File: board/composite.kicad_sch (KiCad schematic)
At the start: 24 parts, among them J10 VGA, J5 VIDEO_JTAG_BYPASS, J6 COMPOSITE, U17 VIDEO, Y1 14.318MHz, Y3 25.175MHz

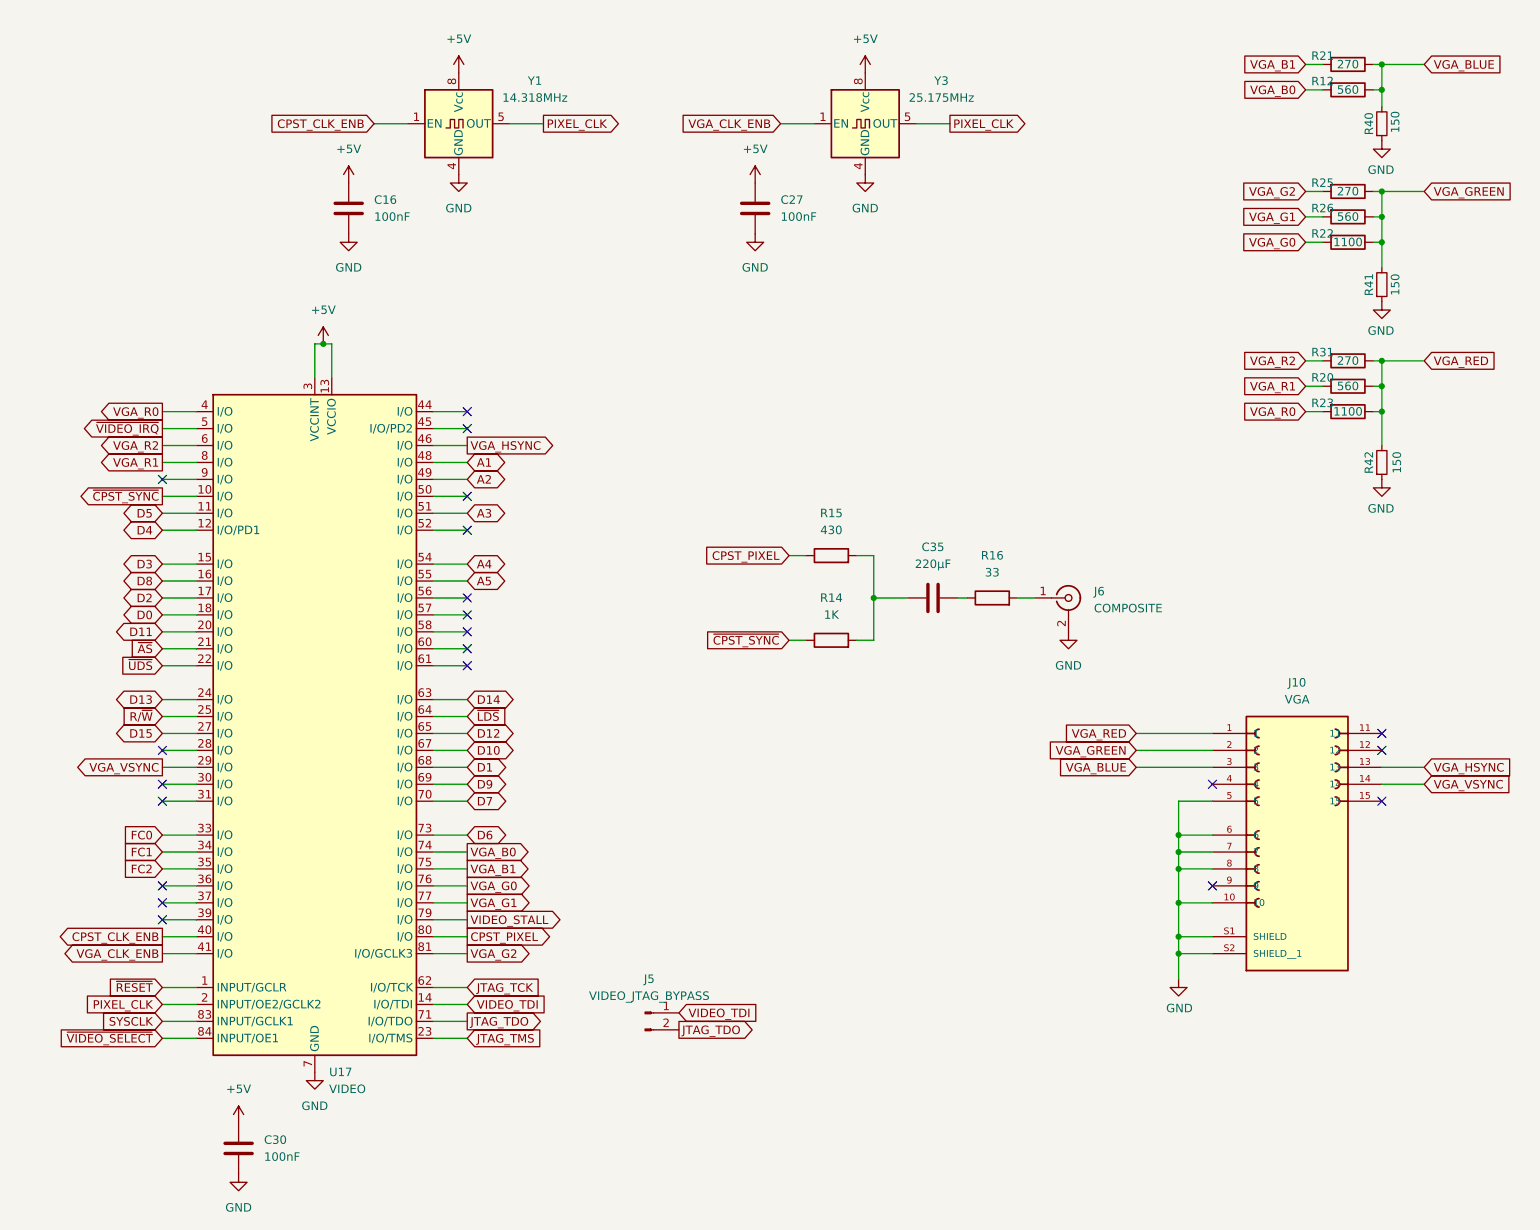
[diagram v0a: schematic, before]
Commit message: update parts I've added
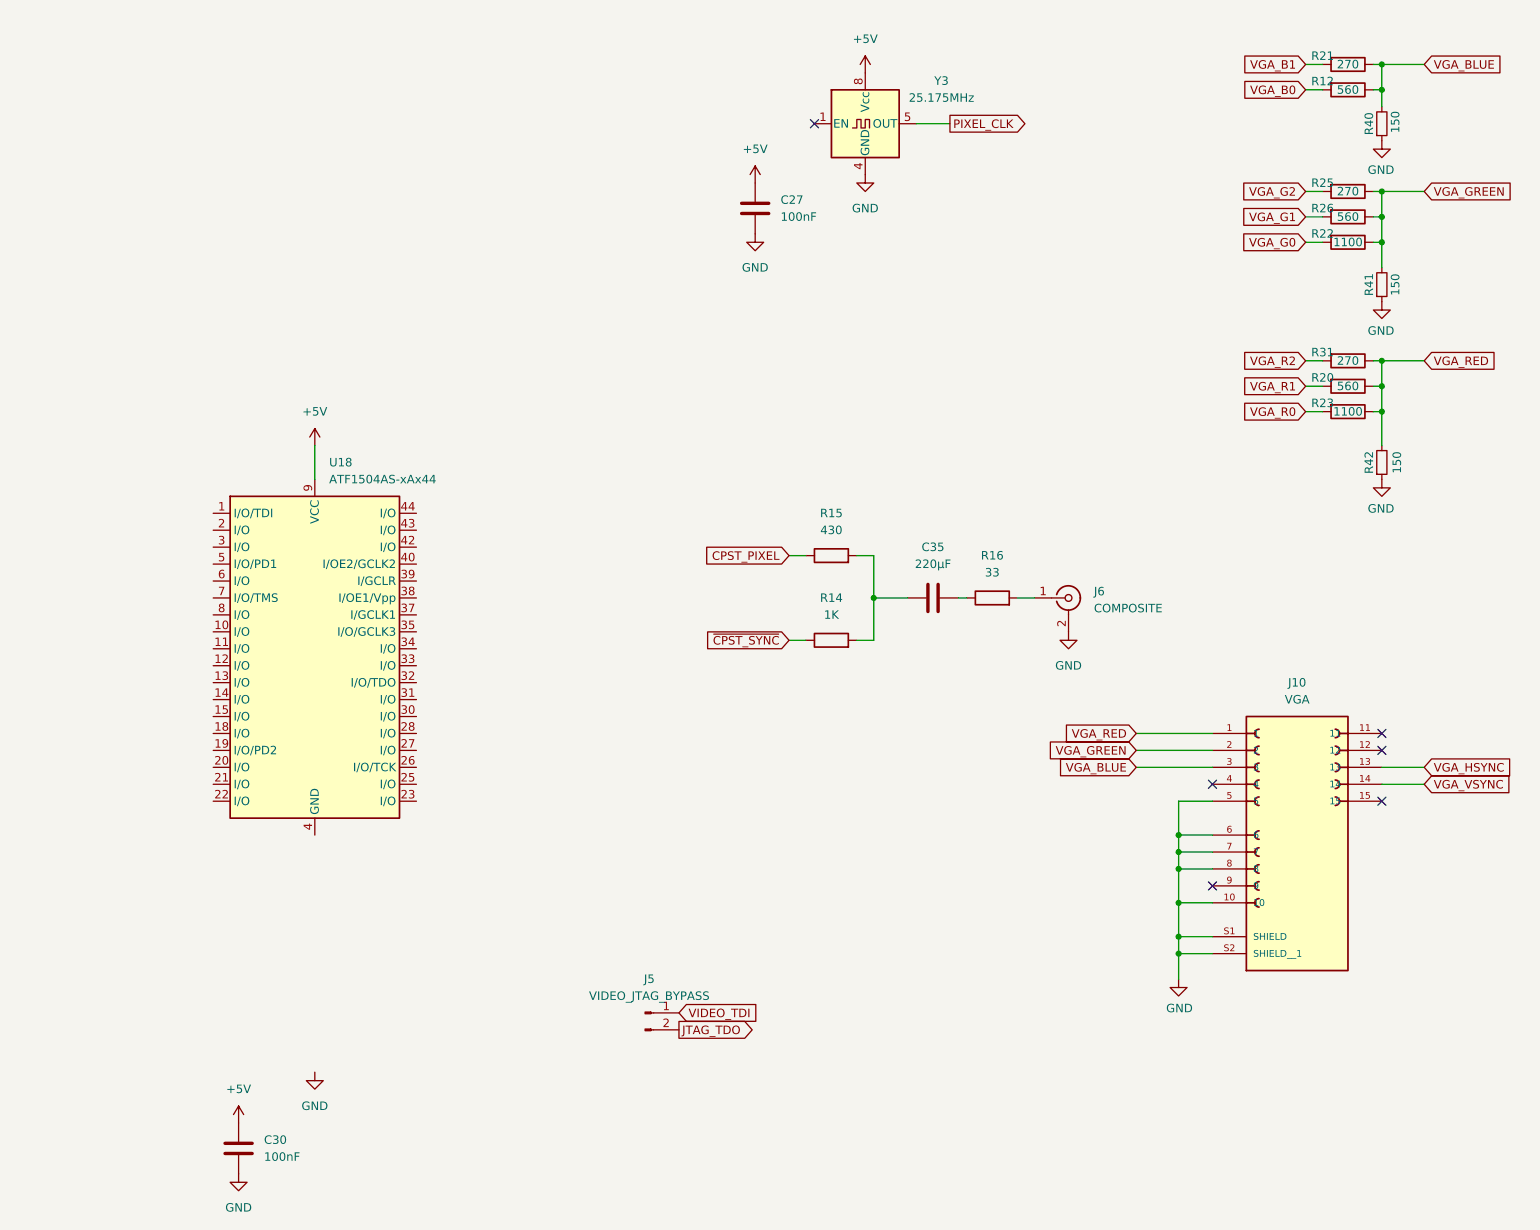
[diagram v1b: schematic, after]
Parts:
- removed C16: 100nF, Capacitor_THT:C_Disc_D5.0mm_W2.5mm_P5.00mm, symbol Device:C
- removed U17: VIDEO, Package_LCC:PLCC-84_THT-Socket, symbol CPLD_Microchip:ATF1508ASx-xxJx84
- removed Y1: 14.318MHz, Oscillator:Oscillator_DIP-8, symbol Oscillator:CXO_DIP8
- added U18: ATF1504AS-xAx44, Package_QFP:TQFP-44_10x10mm_P0.8mm, symbol CPLD_Microchip:ATF1504AS-xAx44
- Y3: Datasheet-rev1 (none) -> http://cdn-reichelt.de/documents/datenblatt/B400/OSZI.pdf; Digikey https://www.digikey.com/en/products/detail/shenzhen-sctf-el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 -> https://www.digikey.com/en/products/detail/ecs-inc/ECS-100A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
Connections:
- net +5V: now also U18.17 (VCC), U18.29 (VCC), U18.41 (VCC), U18.9 (VCC)
- net VGA_CLK_ENB: no longer names the net of Y3.1 (EN)
- new net: U18.16 (GND), U18.24 (GND), U18.36 (GND), U18.4 (GND)
- no-connect marks 21 -> 6

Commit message: checkpoint
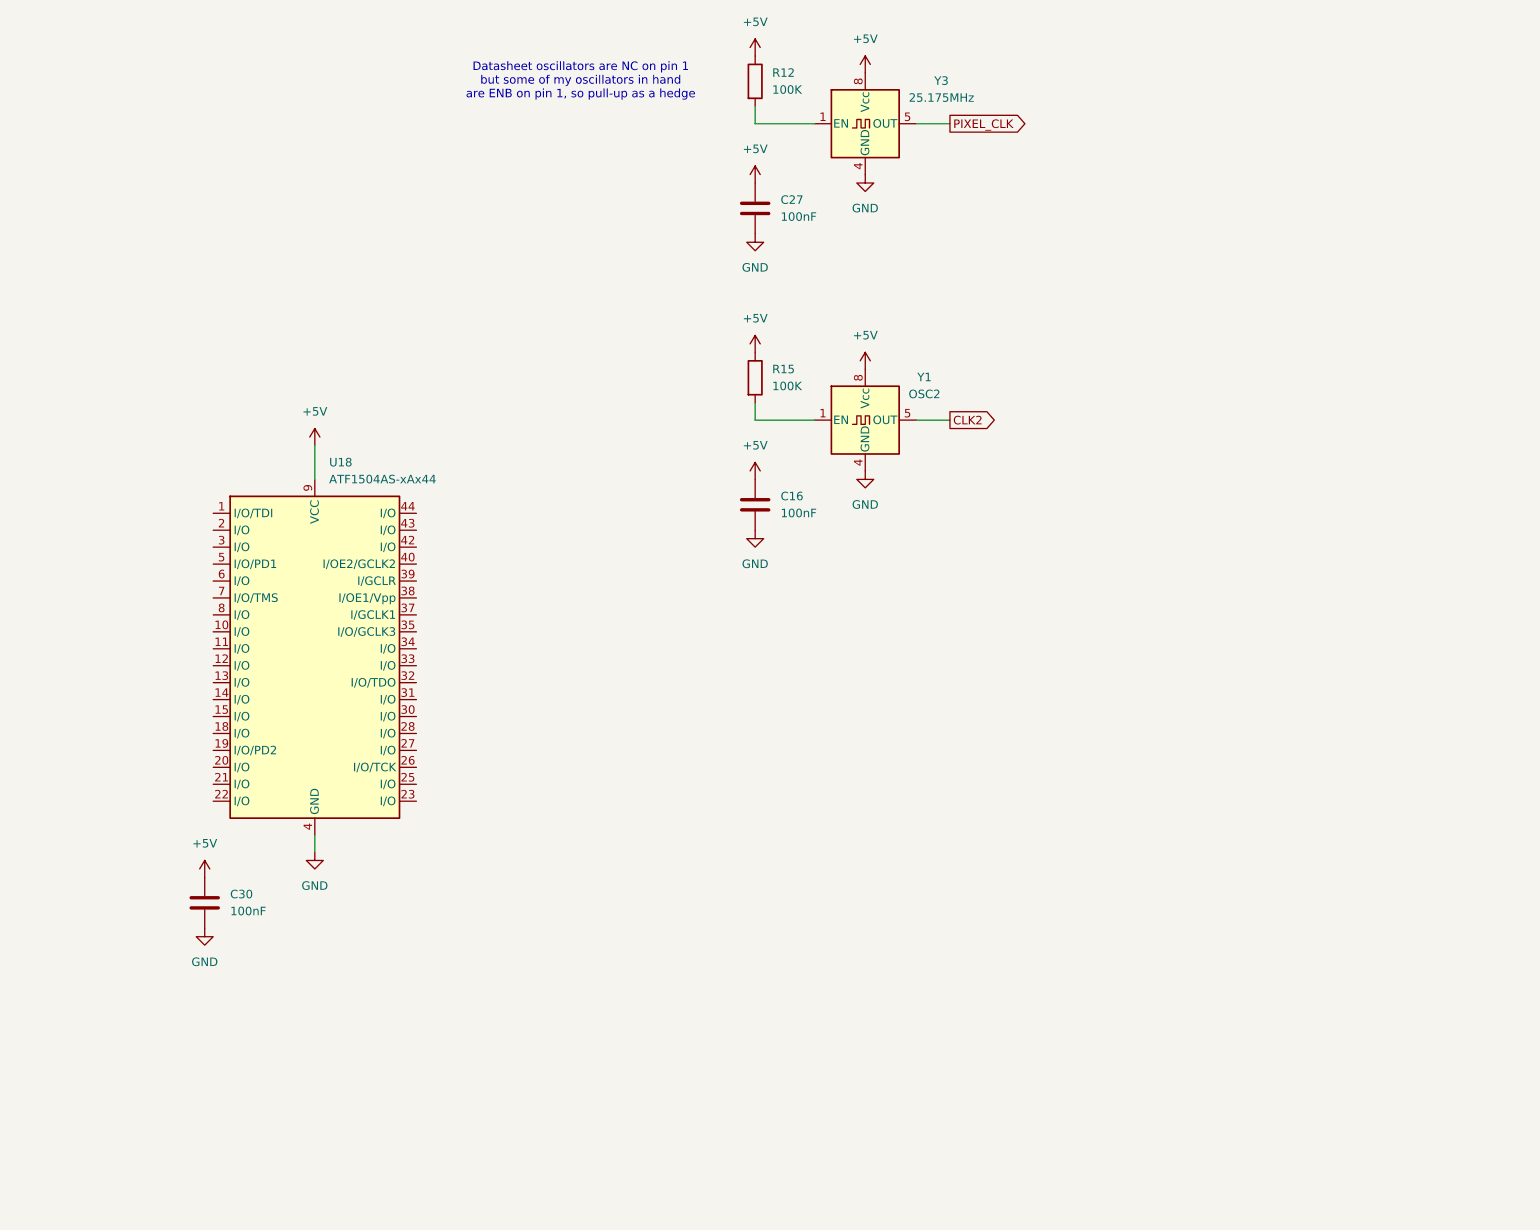
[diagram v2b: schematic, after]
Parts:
- removed C35: 220µF, Capacitor_THT:CP_Radial_D6.3mm_P2.50mm, symbol Device:C
- removed J10: VGA, board:AMPHENOL_ICD15S13E4GX00LF, symbol HD15:ICD15S13E4GX00LF
- removed J5: VIDEO_JTAG_BYPASS, Connector_PinHeader_2.54mm:PinHeader_1x02_P2.54mm_Vertical, symbol Connector:Conn_01x02_Pin
- removed J6: COMPOSITE, board:CUI_RCJ-044, symbol Connector:Conn_Coaxial
- removed R14: 1K, Resistor_THT:R_Axial_DIN0207_L6.3mm_D2.5mm_P10.16mm_Horizontal, symbol Device:R
- removed R16: 33, Resistor_THT:R_Axial_DIN0207_L6.3mm_D2.5mm_P10.16mm_Horizontal, symbol Device:R
- removed R20, R26: 560, Resistor_THT:R_Axial_DIN0207_L6.3mm_D2.5mm_P10.16mm_Horizontal, symbol Device:R
- removed R21, R25, R31: 270, Resistor_THT:R_Axial_DIN0207_L6.3mm_D2.5mm_P10.16mm_Horizontal, symbol Device:R
- removed R22, R23: 1100, Resistor_THT:R_Axial_DIN0207_L6.3mm_D2.5mm_P10.16mm_Horizontal, symbol Device:R
- removed R40, R41, R42: 150, Resistor_THT:R_Axial_DIN0207_L6.3mm_D2.5mm_P10.16mm_Horizontal, symbol Device:R_Small
- added C16: 100nF, Capacitor_THT:C_Disc_D5.0mm_W2.5mm_P5.00mm, symbol Device:C
- added Y1: OSC2, Oscillator:Oscillator_DIP-8, symbol Oscillator:CXO_DIP8
- R12: value 560 -> 100K; Package 0603 -> (none); Type SMD -> (none)
- R15: value 430 -> 100K
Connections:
- net CPST_PIXEL is gone; now on net +5V: R15.1
- net VGA_B0 is gone; now on an unnamed net: R12.2
- net VGA_BLUE is gone; now on net +5V: R12.1
- net +5V: now also C16.1, Y1.8 (Vcc)
- net GND: now also U18.16 (GND), U18.24 (GND), U18.36 (GND), U18.4 (GND), C16.2, Y1.4 (GND)
- net at R15.2: now also Y1.1 (EN)
- new net CLK2: Y1.5 (OUT)
- no-connect marks 6 -> 0
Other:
- note added: "Datasheet oscillators are NC on pin 1 but some of my oscillators in hand are ENB on pin 1, so pull-up as a hedge"
- moved on the sheet: C30
